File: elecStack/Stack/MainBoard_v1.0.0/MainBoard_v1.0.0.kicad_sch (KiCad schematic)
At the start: 28 parts, among them J1 Conn_01x04_Socket, J2 Conn_01x06_Pin, J3 Conn_01x06_Pin, J4 Conn_01x20_Socket, J5 Conn_01x20_Socket, Q1 NMOS, Q2 NMOS, Q3 NMOS, Q4 NMOS, Q5 NMOS, Q6 NMOS, Q7 NMOS, Q8 PMOS, U1 RASPBERRY_PI_PICO, U2 L293D, U3 TXS0108EPW, U4 L293D

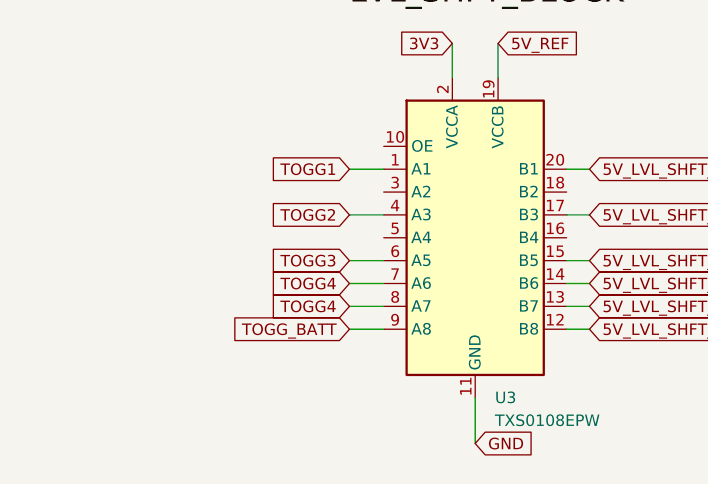
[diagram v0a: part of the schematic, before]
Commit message: Updated version 1
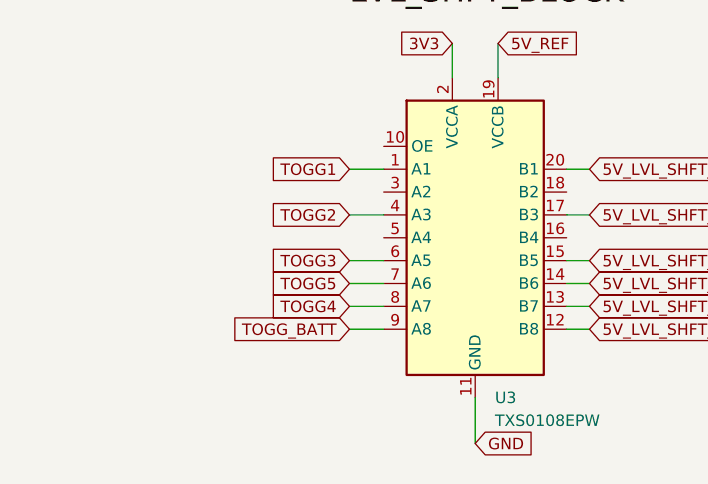
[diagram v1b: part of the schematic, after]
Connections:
- net TOGG4: no longer U3.7 (A6)
- new net TOGG5: U3.7 (A6)
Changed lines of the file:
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@@
 		)
 	)
-	(global_label "TOGG4"
+	(global_label "TOGG5"
 		(shape input)
 		(at 46.99 177.8 180)
